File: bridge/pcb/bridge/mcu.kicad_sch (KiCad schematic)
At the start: 12 parts, among them Q1 PMOS, Q2 PMOS, Q3 PMOS, Q4 PMOS, Q5 PMOS, U1 YAAJ_BluePill

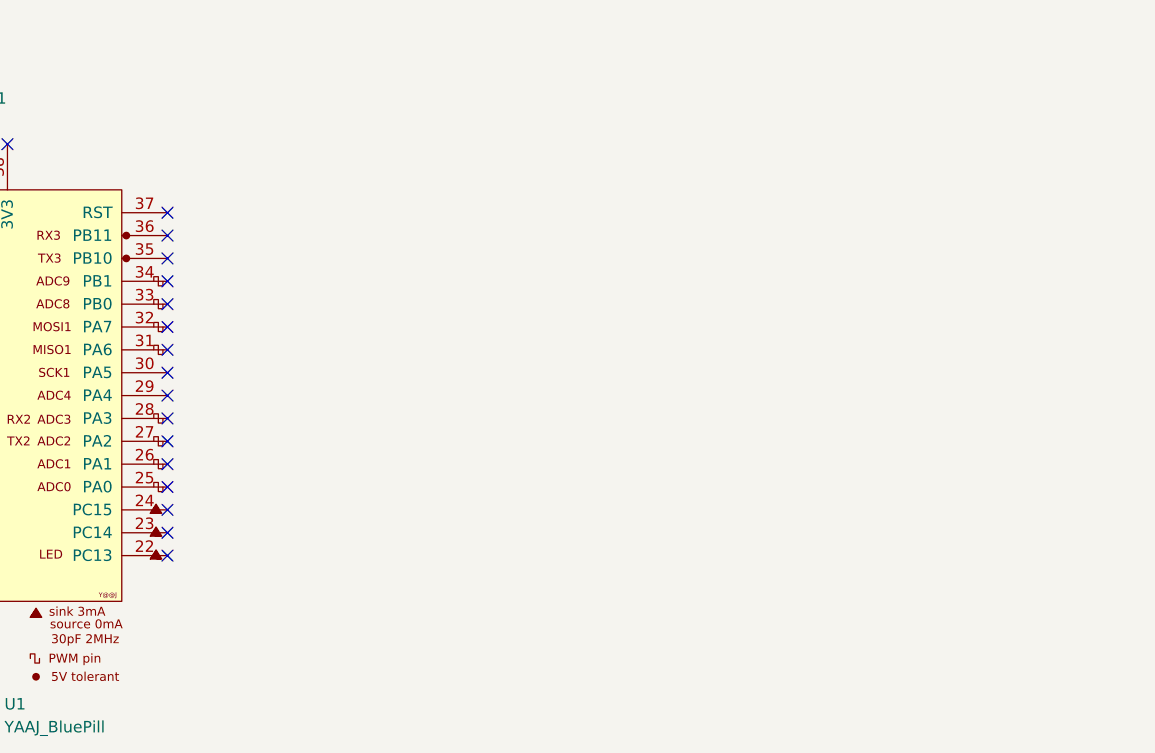
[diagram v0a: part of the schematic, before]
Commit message: Fixed issues, added DAC
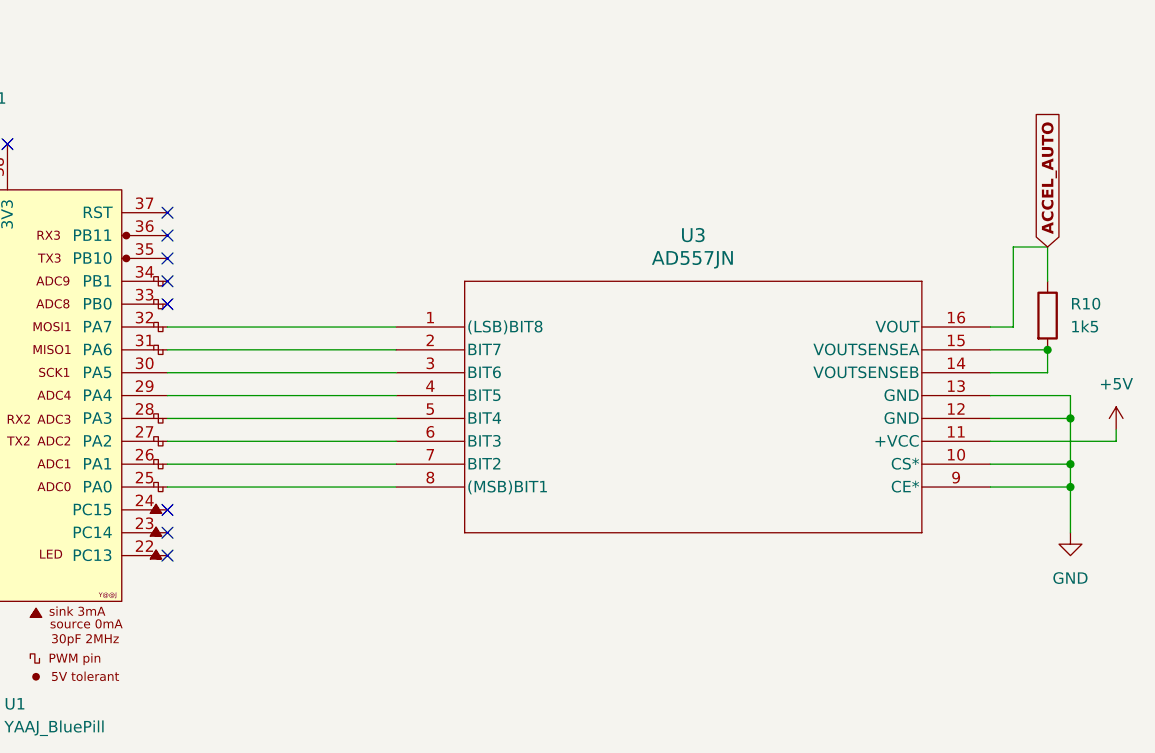
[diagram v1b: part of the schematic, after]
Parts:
- added R10: 1k5, Resistor_THT:R_Axial_DIN0309_L9.0mm_D3.2mm_P12.70mm_Horizontal, symbol Device:R
- added U3: AD557JN, bridge:AD557JN, symbol bridge:AD557JN
- Q1, Q2, Q3, Q4, Q5: footprint Package_TO_SOT_THT:TO-3P-3_Horizontal_TabDown -> Package_TO_SOT_THT:TO-220-3_Horizontal_TabDown
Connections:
- net +5V: now also U3.11 (+VCC)
- net GND: now also U3.10 (CS*), U3.12 (GND), U3.13 (GND), U3.9 (CE*)
- net at U1.25 (PA0): now also U3.8 ((MSB)BIT1)
- net at U1.26 (PA1): now also U3.7 (BIT2)
- net at U1.27 (PA2): now also U3.6 (BIT3)
- net at U1.28 (PA3): now also U3.5 (BIT4)
- net at U1.29 (PA4): now also U3.4 (BIT5)
- net at U1.30 (PA5): now also U3.3 (BIT6)
- net at U1.31 (PA6): now also U3.2 (BIT7)
- net at U1.32 (PA7): now also U3.1 ((LSB)BIT8)
- new net: R10.2, U3.14 (VOUTSENSEB), U3.15 (VOUTSENSEA)
- new net ACCEL_AUTO: R10.1, U3.16 (VOUT)
- no-connect marks 30 -> 22

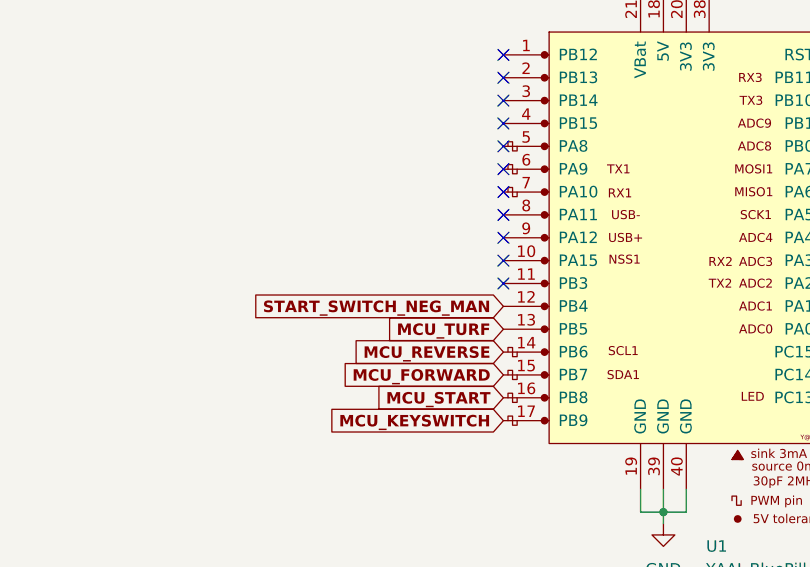
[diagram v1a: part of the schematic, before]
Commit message: Completed schematic
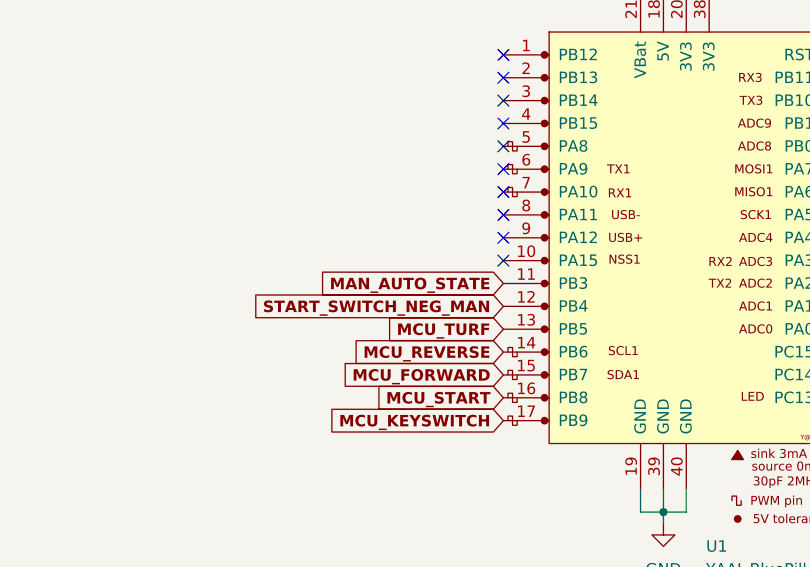
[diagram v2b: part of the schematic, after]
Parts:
- R1, R10, R2, R3, R4, R5: footprint Resistor_THT:R_Axial_DIN0309_L9.0mm_D3.2mm_P12.70mm_Horizontal -> bridge:THT_RESISTOR_WITH_VALUE
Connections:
- net MAN_AUTO_STATE: now reaches U1.11 (PB3)
- no-connect marks 22 -> 21
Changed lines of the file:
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@@
   (no_connect (at 130.81 46.99))
   (no_connect (at 90.17 57.15))
-  (no_connect (at 90.17 64.77))
   (no_connect (at 130.81 74.93))
   (no_connect (at 130.81 44.45))
@@
     )
   )
+  (global_label "MAN_AUTO_STATE" (shape input) (at 90.17 64.77 180) (fields_autoplaced)
+    (effects (font (size 1.27 1.27) bold) (justify right))
+    (property "Intersheetrefs" "${INTERSHEET_REFS}" (at 70.8036 64.77 0)
+      (effects (font (size 1.27 1.27)) (justify right) hide)
+    )
+  )
   (global_label "MCU_START" (shape input) (at 57.15 162.56 0) (fields_autoplaced)
     (effects (font (size 1.27 1.27) (thickness 0.254) bold) (justify left))
@@
       (effects (font (size 1.27 1.27)))
     )
-    (property "Footprint" "Resistor_THT:R_Axial_DIN0309_L9.0mm_D3.2mm_P12.70mm_Horizontal" (at 53.34 164.338 90)
+    (property "Footprint" "bridge:THT_RESISTOR_WITH_VALUE" (at 53.34 164.338 90)
       (effects (font (size 1.27 1.27)) hide)
     )
@@
       (effects (font (size 1.27 1.27)))
     )
-    (property "Footprint" "Resistor_THT:R_Axial_DIN0309_L9.0mm_D3.2mm_P12.70mm_Horizontal" (at 53.34 130.048 90)
+    (property "Footprint" "bridge:THT_RESISTOR_WITH_VALUE" (at 53.34 130.048 90)
       (effects (font (size 1.27 1.27)) hide)
     )
@@
       (effects (font (size 1.27 1.27)))
     )
-    (property "Footprint" "Resistor_THT:R_Axial_DIN0309_L9.0mm_D3.2mm_P12.70mm_Horizontal" (at 114.3 164.338 90)
+    (property "Footprint" "bridge:THT_RESISTOR_WITH_VALUE" (at 114.3 164.338 90)
       (effects (font (size 1.27 1.27)) hide)
     )
@@
       (effects (font (size 1.27 1.27)) (justify left))
     )
-    (property "Footprint" "Resistor_THT:R_Axial_DIN0309_L9.0mm_D3.2mm_P12.70mm_Horizontal" (at 226.822 50.8 90)
+    (property "Footprint" "bridge:THT_RESISTOR_WITH_VALUE" (at 226.822 50.8 90)
       (effects (font (size 1.27 1.27)) hide)
     )
@@
       (effects (font (size 1.27 1.27)))
     )
-    (property "Footprint" "Resistor_THT:R_Axial_DIN0309_L9.0mm_D3.2mm_P12.70mm_Horizontal" (at 142.24 126.238 90)
+    (property "Footprint" "bridge:THT_RESISTOR_WITH_VALUE" (at 142.24 126.238 90)
       (effects (font (size 1.27 1.27)) hide)
     )
@@
       (effects (font (size 1.27 1.27)))
     )
-    (property "Footprint" "Resistor_THT:R_Axial_DIN0309_L9.0mm_D3.2mm_P12.70mm_Horizontal" (at 161.29 164.338 90)
-      (effects (font (size 1.27 1.27)) hide)
-    )
+    (property "Footprint" "bridge:THT_RESISTOR_WITH_VALUE" (at 161.29 164.338 90)
+      (effects (font (size 1.27 1.27)) hide)
+    )
